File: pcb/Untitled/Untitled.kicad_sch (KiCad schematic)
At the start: 30 parts, among them J1 Conn_01x09, J2 Micro_SD_Card_Det1, J3 USB_C_Receptacle_USB2.0_14P, J4 Conn_01x02, J5 Conn_Coaxial, Q1 FS8205A, Q2 AO3407A, SW1 SW_Push, SW2 SW_Push, SW3 SW_Push, SW4 SW_Push, SW5 SW_Push, SW6 SW_Push, SW7 SW_Push, SW8 SW_Push, SW9 SW_Push, U1 ESP32-S3-WROOM-1, U10 RV-3028-C8-32.768KHZ-1PPM-TA-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, U2 MAX-M10S, U3 USBLC6-2SC6, U4 MCP73831-2-MC, U5 AP2112K-3.3, U6 DW01A, U7 LIS3MDL, U8 BMP390, U9 SHT4x

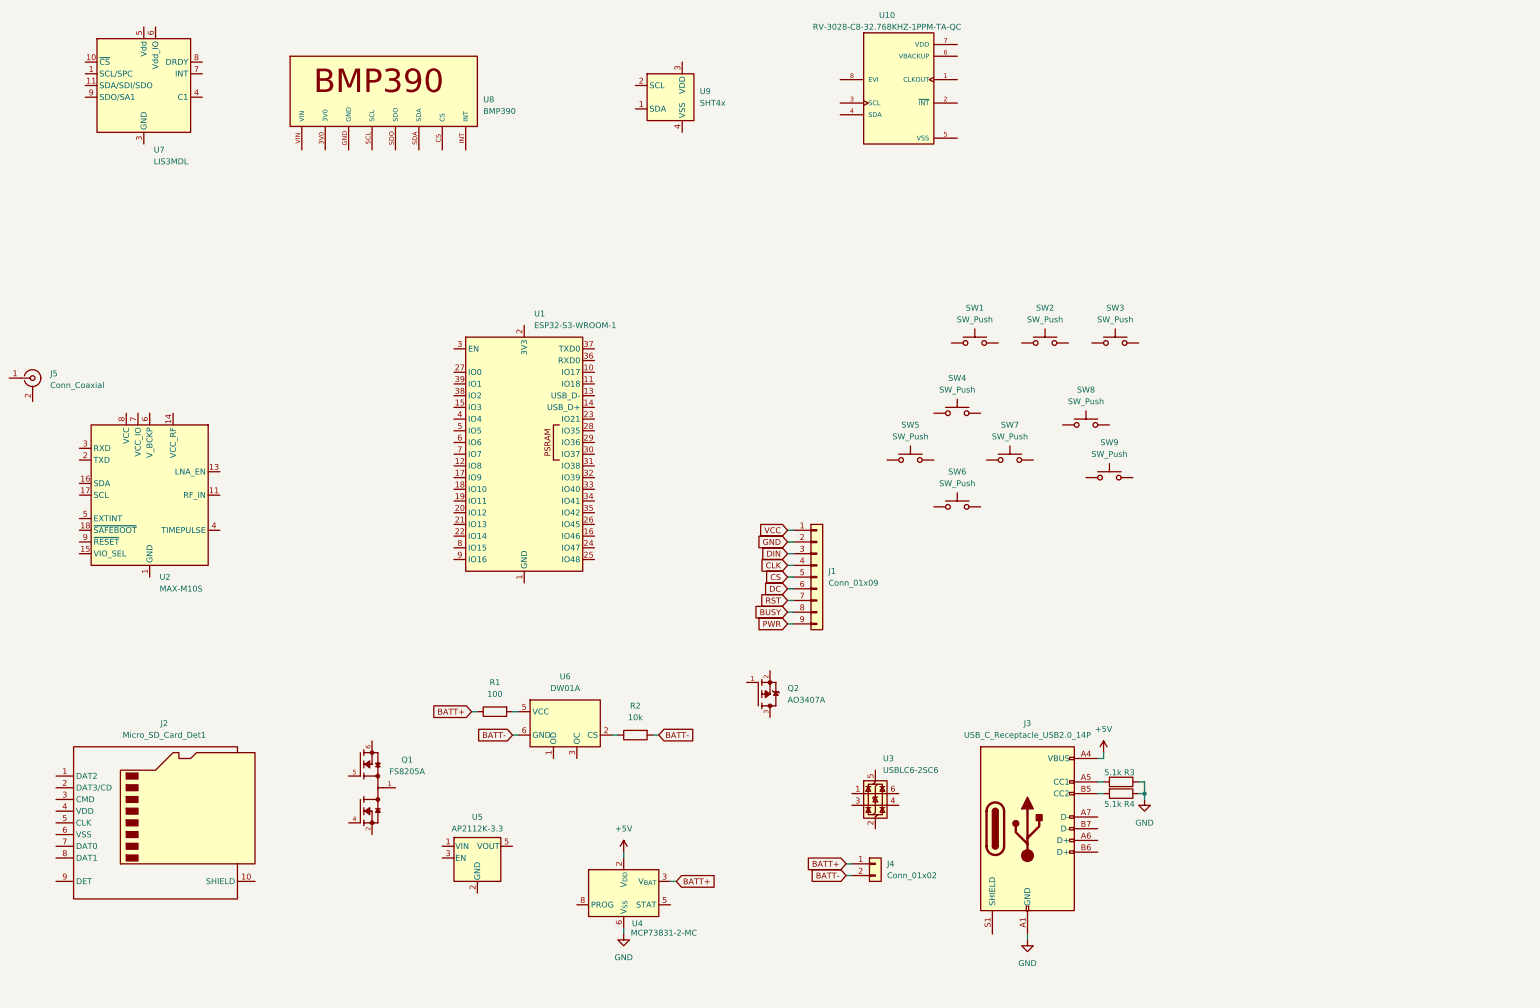
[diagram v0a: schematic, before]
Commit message: boop
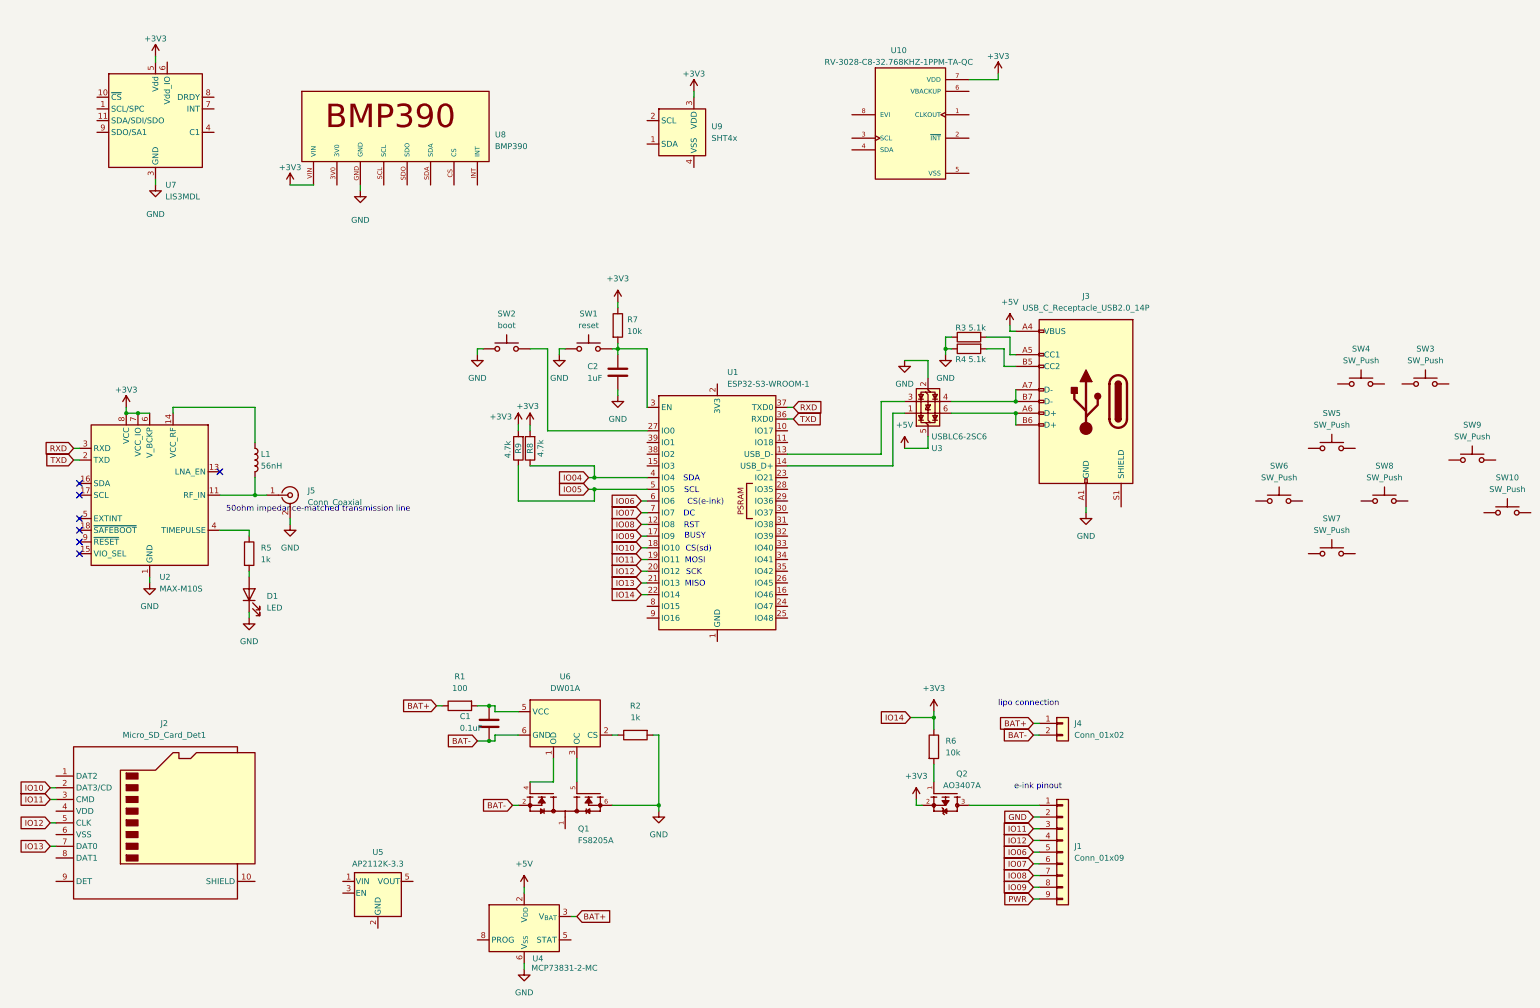
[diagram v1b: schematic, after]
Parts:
- added C1: 0.1uF, symbol Device:C
- added C2: 1uF, symbol Device:C
- added D1: LED, symbol Device:LED
- added L1: 56nH, symbol Device:L
- added R5: 1k, symbol Device:R
- added R6, R7: 10k, symbol Device:R
- added R8, R9: 4.7k, symbol Device:R
- added SW10: SW_Push, symbol Switch:SW_Push
- R2: value 10k -> 1k
- SW1: value SW_Push -> reset
- SW2: value SW_Push -> boot
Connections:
- net BUSY is gone; now on net IO09: J1.8 (Pin_8)
- net CLK is gone; now on net IO12: J1.4 (Pin_4)
- net CS is gone; now on net IO06: J1.5 (Pin_5)
- net DC is gone; now on net IO07: J1.6 (Pin_6)
- net DIN is gone; now on net IO11: J1.3 (Pin_3)
- net RST is gone; now on net IO08: J1.7 (Pin_7)
- net VCC is gone; now on an unnamed net: J1.1 (Pin_1)
- net +5V: now also U3.5 (VBUS)
- net GND: now also J5.2 (Ext), Q1.6, Q1.7, R2.2, SW1.1, SW2.1, U2.1 (GND), U2.10 (GND), U2.12 (GND), U3.2 (GND), U7.12 (GND), U7.2 (GND), U7.3 (GND), U8.GND, C2.2, D1.1 (K)
- net at R1.2, U6.5 (VCC): now also C1.1
- net IO08: now reaches U1.12 (IO8)
- net at U1.13 (USB_D-): now also U3.3 (I/O2)
- net at U1.14 (USB_D+): now also U3.1 (I/O1)
- net IO09: now reaches U1.17 (IO9)
- net IO10: now reaches U1.18 (IO10)
- net IO10: now also J2.2 (DAT3/CD)
- net IO11: now reaches U1.19 (IO11)
- net IO11: now also J2.3 (CMD)
- net IO12: now reaches U1.20 (IO12)
- net IO12: now also J2.5 (CLK)
- net IO13: now reaches U1.21 (IO13)
- net IO13: now also J2.7 (DAT0)
- net +3V3: now reaches U1.22 (IO14)
- net +3V3: now also Q2.2, U10.7 (VDD), U2.6 (V_BCKP), U2.7 (VCC_IO), U2.8 (VCC), U7.5 (Vdd), U8.VIN, U9.3 (VDD), R6.1, R7.1, R8.2, R9.2
- net at U1.27 (IO0): now also SW2.2
- net at U1.3 (EN): now also SW1.2, C2.1, R7.2
- net TXD: now reaches U1.36 (RXD0)
- net TXD: now also U2.2 (TXD)
- net RXD: now reaches U1.37 (TXD0)
- net RXD: now also U2.3 (RXD)
- net IO04: now reaches U1.4 (IO4)
- net IO04: now also R8.1
- net IO05: now reaches U1.5 (IO5)
- net IO05: now also R9.1
- net IO06: now reaches U1.6 (IO6)
- net IO07: now reaches U1.7 (IO7)
- net at J3.A6 (D+): now also J3.B6 (D+), U3.6 (I/O1)
- net at J3.A7 (D-): now also J3.B7 (D-), U3.4 (I/O2)
- net at U2.11 (RF_IN): now also J5.1 (In), L1.2
- net at U2.14 (VCC_RF): now also L1.1
- net at U2.4 (TIMEPULSE): now also R5.1
- net BAT-: now reaches Q1.2, Q1.3
- net BAT-: now also J4.2 (Pin_2), U6.6 (GND), C1.2
- net at Q1.4: now also U6.1 (OD)
- net at Q1.5: now also U6.3 (OC)
- net at Q2.1: now also R6.2
- net BATT+ renamed BAT+
- removed net BATT-: J4.2 (Pin_2), R2.2, U6.6 (GND)
- new net: D1.2 (A), R5.2
- no-connect marks 0 -> 7
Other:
- note added: "50ohm impedance-matched transmission line"
- note added: "BUSY"
- note added: "CS(e-ink)"
- note added: "CS(sd)"
- note added: "DC"
- note added: "MISO"
- note added: "MOSI"
- note added: "RST"
- note added: "SCK"
- note added: "SCL"
- note added: "SDA"
- note added: "e-ink pinout"
- note added: "lipo connection"
- moved on the sheet: J1, J3, J4, J5, Q1, Q2, R1, R3, R4, SW1, SW2, SW3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
